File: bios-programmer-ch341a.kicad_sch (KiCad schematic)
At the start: 49 parts, among them J1 USB_B_Micro, J2 SPI Debug, J3 I²C Debug, J4 -Banana-, J5 +Banana+, J6 ZIF16, J7 Conn_02x04_Counter_Clockwise, J8 Conn_02x04_Counter_Clockwise, Q1 SSM3J328R, Q2 SSM3J328R, Q3 SSM3J328R, Q4 SSM3J328R, SW1 RESET, U1 CH341A, U2 ISO6741, U3 ADuM1252, U4 TL432DBZ, Y1 12MHz

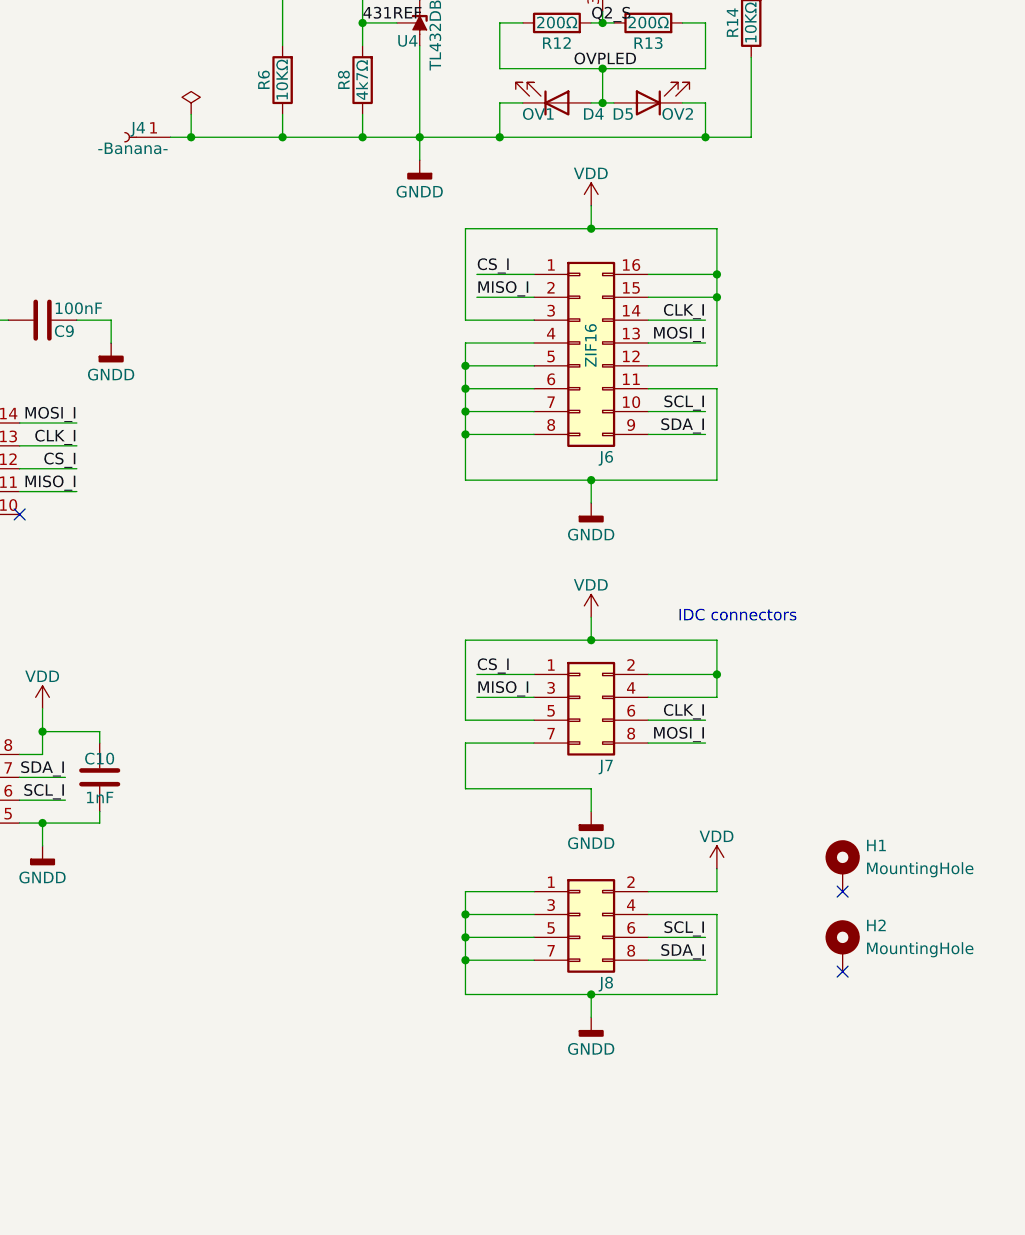
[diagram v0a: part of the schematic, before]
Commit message: adding sense wires; beautification; issue with 2x05 IDC connector on top of isolator to be fixed
PCB temp bijna sense zonde bovenkant

pcb sense on bottom done; cleanup todo
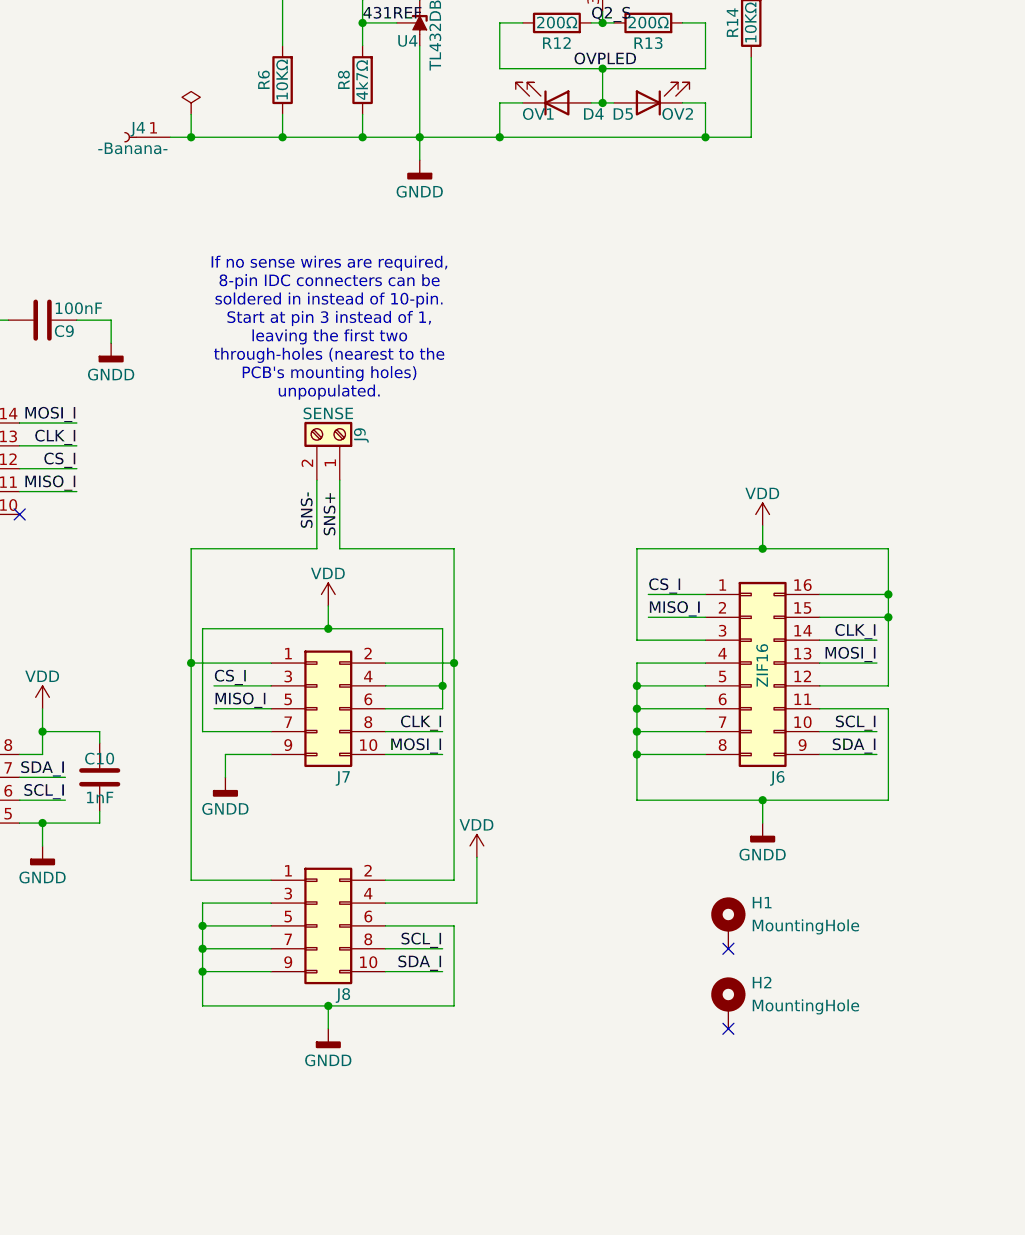
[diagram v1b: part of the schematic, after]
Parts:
- added J9: SENSE, TerminalBlock_TE-Connectivity:TerminalBlock_TE_282834-2_1x02_P2.54mm_Horizontal, symbol Connector:Screw_Terminal_01x02
- J7, J8: value Conn_02x04_Counter_Clockwise -> Conn_02x05_Odd_Even; footprint Connector_IDC:IDC-Header_2x04_P2.54mm_Horizontal -> footprints:IDC-Header_2x05_P2.54mm_Horizontal_1.64mm_pad; symbol Connector_Generic:Conn_02x04_Odd_Even -> Connector_Generic:Conn_02x05_Odd_Even
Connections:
- net CLK_I: now also J7.8 (Pin_8); no longer J7.6 (Pin_6)
- net CS_I: now also J7.3 (Pin_3); no longer J7.1 (Pin_1)
- net GNDD: now also J7.9 (Pin_9), J8.6 (Pin_6), J8.9 (Pin_9); no longer J7.7 (Pin_7), J8.1 (Pin_1), J8.4 (Pin_4)
- net MISO_I: now also J7.5 (Pin_5); no longer J7.3 (Pin_3)
- net MOSI_I: now also J7.10 (Pin_10); no longer J7.8 (Pin_8)
- net SCL_I: now also J8.8 (Pin_8); no longer J8.6 (Pin_6)
- net SDA_I: now also J8.10 (Pin_10); no longer J8.8 (Pin_8)
- net VDD: now also J7.6 (Pin_6), J7.7 (Pin_7), J8.4 (Pin_4); no longer J7.2 (Pin_2), J7.5 (Pin_5), J8.2 (Pin_2)
- new net SNS+: J7.2 (Pin_2), J8.2 (Pin_2), J9.1 (Pin_1)
- new net SNS-: J7.1 (Pin_1), J8.1 (Pin_1), J9.2 (Pin_2)
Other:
- note removed: "IDC connectors"
- moved on the sheet: H1, H2, J6
